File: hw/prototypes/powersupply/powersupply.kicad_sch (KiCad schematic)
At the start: 55 parts, among them J1 Conn_01x02_Pin, J2 Conn_01x02_Pin, J3 Conn_01x03_Pin, J4 Conn_01x03_Pin, U1 SN6507DGQ, U2 LT3042xMSE, U3 LT3093xMSE, U4 TPS7A39

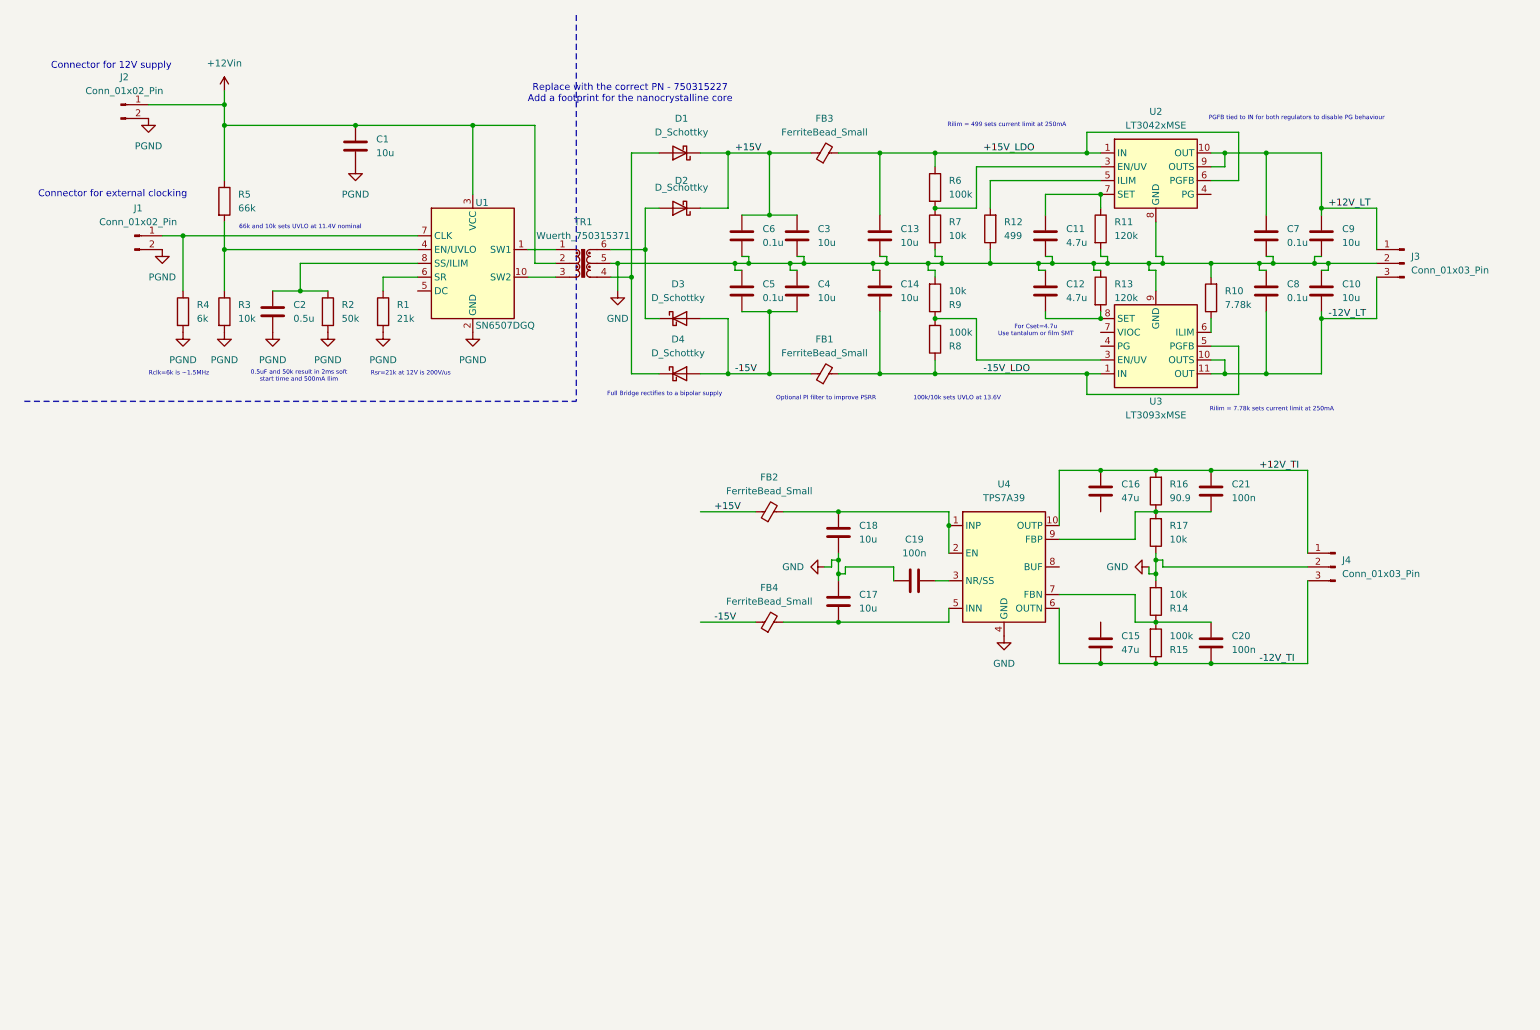
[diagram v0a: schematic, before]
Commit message: Pushing old changes
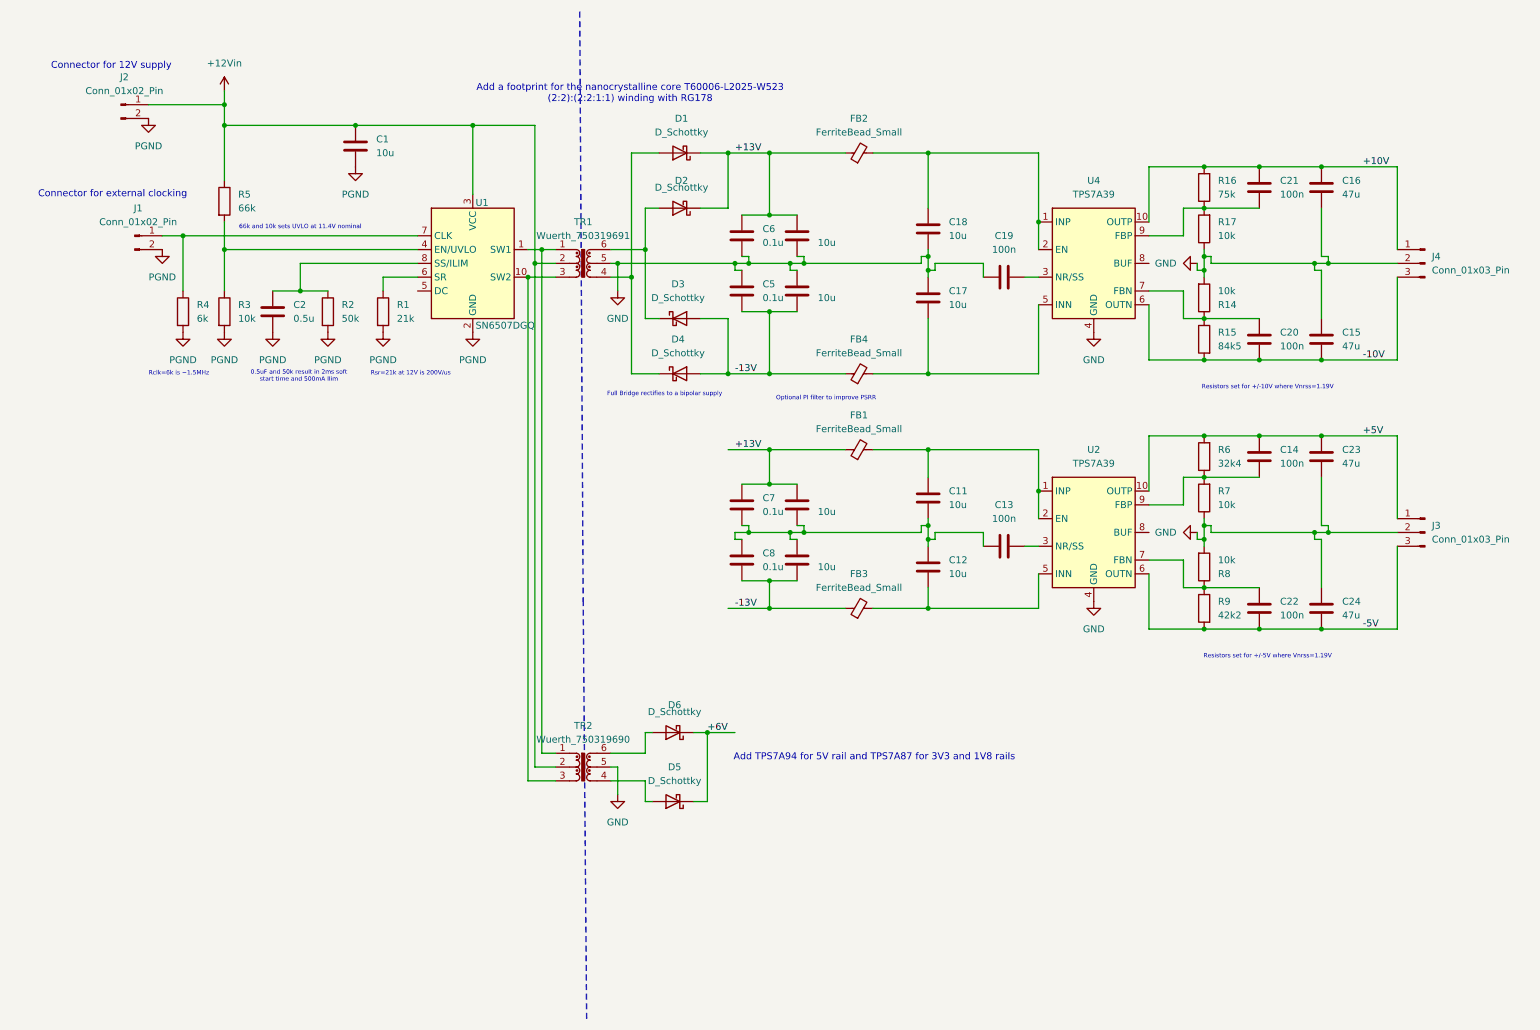
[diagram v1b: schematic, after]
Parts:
- removed R10: 7.78k, symbol Device:R
- removed R11, R13: 120k, symbol Device:R
- removed R12: 499, symbol Device:R
- removed U2: LT3042xMSE, Package_SO:MSOP-10-1EP_3x3mm_P0.5mm_EP1.68x1.88mm, symbol Regulator_Linear:LT3042xMSE
- removed U3: LT3093xMSE, Package_SO:MSOP-12-1EP_3x4mm_P0.65mm_EP1.65x2.85mm, symbol Regulator_Linear:LT3093xMSE
- added C22: 100n, symbol Device:C
- added C23, C24: 47u, symbol Device:C
- added D5, D6: D_Schottky, symbol Device:D_Schottky
- added TR2: Wuerth_750319690, Transformer_SMD:Transformer_Wuerth_750315371, symbol Transformer:Wuerth_750315371
- added U2: TPS7A39, Package_SON:Texas_S-PVSON-N10_ThermalVias, symbol Regulator_Linear:TPS7A39
- C11, C12: value 4.7u -> 10u
- C13, C14: value 10u -> 100n
- R15: value 100k -> 84k5
- R16: value 90.9 -> 75k
- R6: value 100k -> 32k4
- R8: value 100k -> 10k
- R9: value 10k -> 42k2
- TR1: value Wuerth_750315371 -> Wuerth_750319691
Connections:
- net +12Vin: now also TR2.2
- net GND: now also C15.1, C16.2, R7.1, R8.2, C23.2, C24.1, TR2.5, U2.11 (GND), U2.4 (GND); no longer C10.1, C11.2, C12.1, C13.2, C14.1, C7.2, C8.1, C9.2, R7.2, R9.2
- net at R9.1: now also R8.1, C22.1, U2.7 (FBN); no longer R8.2
- net at C11.1: now also FB1.2, U2.1 (INP), U2.2 (EN)
- net at C12.2: now also FB3.2, U2.5 (INN)
- net +5V: now reaches R6.2
- net +5V: now also C14.1, J3.1 (Pin_1), C23.1, U2.10 (OUTP); no longer R7.1
- net at C20.1, R14.1, U4.7 (FBN): now also R15.1; no longer R15.2
- net at TR1.1, U1.1 (SW1): now also TR2.1
- net at TR1.3, U1.10 (SW2): now also TR2.3
- net +12V_LT renamed +13V
- net +13V: now also C3.1, C6.1, D1.1 (K), D2.1 (K), FB1.1, FB2.1; no longer J3.1 (Pin_1)
- net +12V_TI renamed +10V
- removed net +15V: C3.1, C6.1, D1.1 (K), D2.1 (K), FB2.1, FB3.1
- removed net +15V_LDO: C13.1, FB3.2, R6.1
- net -12V_LT renamed -13V
- net -13V: now also C4.2, C5.2, D3.2 (A), D4.2 (A), FB3.1, FB4.1; no longer J3.3 (Pin_3)
- net -12V_TI renamed -10V
- net -10V: now also R15.2; no longer R15.1
- removed net -15V: C4.2, C5.2, D3.2 (A), D4.2 (A), FB1.1, FB4.1
- removed net -15V_LDO: C14.2, FB1.2, R8.1
- new net: C10.1, C11.2, C12.1, C13.2, C7.2, C8.1, C9.2
- new net: C14.2, R6.1, R7.2, U2.9 (FBP)
- new net: D5.2 (A), TR2.4
- new net: D6.2 (A), TR2.6
- new net: C13.1, U2.3 (NR/SS)
- new net +6V: D5.1 (K), D6.1 (K)
- new net -5V: C22.2, C24.2, J3.3 (Pin_3), R9.2, U2.6 (OUTN)
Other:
- note added: "Add TPS7A94 for 5V rail and TPS7A87 for 3V3 and 1V8 rails"
- note added: "Add a footprint for the nanocrystalline core T60006-L2025-W523 (2:2):(2:2:1:1) winding with RG178"
- note added: "Resistors set for +/-10V where Vnrss=1.19V"
- note added: "Resistors set for +/-5V where Vnrss=1.19V"
- note removed: "100k/10k sets UVLO at 13.6V"
- note removed: "For Cset=4.7u Use tantalum or film SMT"
- note removed: "PGFB tied to IN for both regulators to disable PG behaviour"
- note removed: "Replace with the correct PN - 750315227 Add a footprint for the nanocrystalline core"
- note removed: "Rilim = 499 sets current limit at 250mA"
- note removed: "Rilim = 7.78k sets current limit at 250mA"
- moved on the sheet: C15, C16, C17, C18, C19, C20, C21, FB2, FB4, J4, R14, R15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
